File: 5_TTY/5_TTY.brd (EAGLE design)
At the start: 67.4 x 44.8 mm, 29 parts, among them Q2 BC857C, Q3 BC857C, Q4 BC857C, Q5 BC857C, Q6 BC857C, T4 BC847, X1 ALLSERIALSLAVE, X7 AKL18X-04W

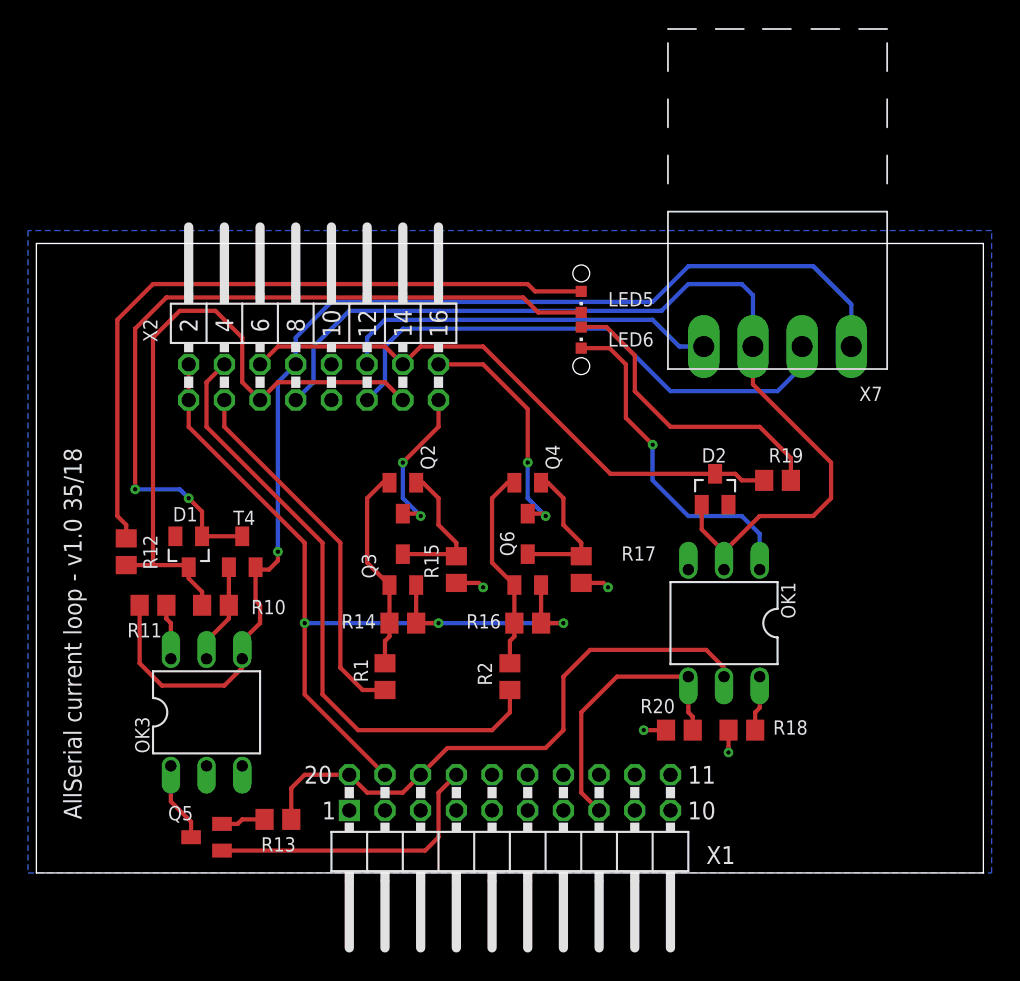
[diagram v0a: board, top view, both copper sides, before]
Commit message: final design & order
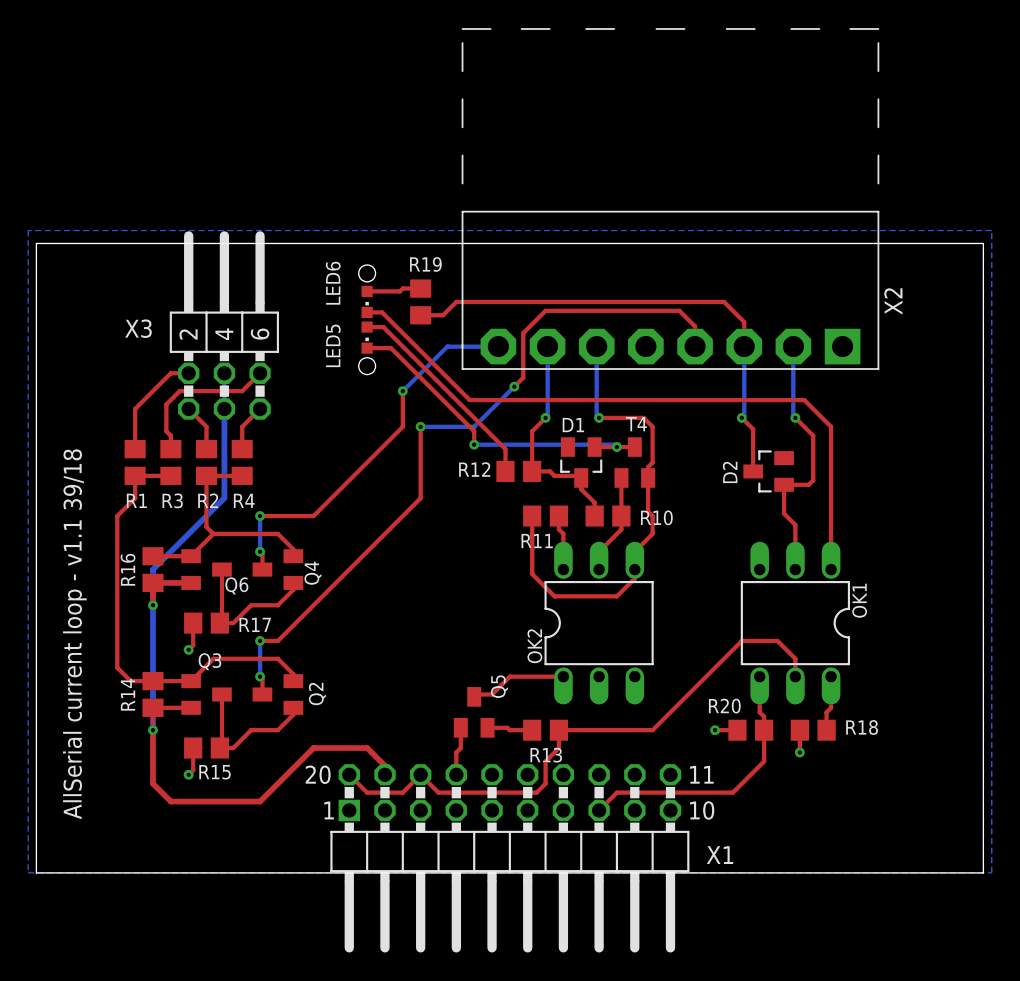
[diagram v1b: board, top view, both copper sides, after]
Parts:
- removed OK3: 4N25, optocoupler:DIL06
- removed X7: AKL18X-04W, con-riacon_akl:AKL182-04
- added OK2: 4N25, optocoupler:DIL06
- added R3, R4: 68R, resistor:R0805
- added X3: MA03-2W, con-lstb:MA03-2W
- R1, R2: value 33R -> 15R
- R14: value 33R -> 68R
- X2: value (none) -> AKL18X-08W; device con-lstb:MA08-2W -> con-riacon_akl:AKL182-08
- moved D1 28.7 mm to (39.4, 29.2)
- moved R10 28.7 mm to (41.3, 25.4)
- moved R11 28.7 mm to (36.8, 25.4)
- moved T4 28.7 mm to (43.2, 29.2)
- moved R12 28.5 mm to (34.9, 28.6), turned to 180 degrees
- moved R19 28.4 mm to (27.9, 40.6), turned to 90 degrees
- moved R16 26.9 mm to (8.89, 21.6), turned to 90 degrees
- moved R17 26.9 mm to (12.7, 17.8), turned to 0 degrees
- moved R2 26.4 mm to (12.7, 29.2), turned to 270 degrees
- moved X2 25.5 mm to (45.7, 37.5), turned to 180 degrees
- moved R1 23.4 mm to (7.62, 29.2), turned to 270 degrees
- moved Q6 22.9 mm to (12.7, 21.6), turned to 270 degrees
- moved R15 21.8 mm to (12.7, 8.89), turned to 0 degrees
- moved Q5 21.0 mm to (31.8, 11.4), turned to 0 degrees
- moved R13 20.1 mm to (36.8, 10.2)
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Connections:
- removed net CS1: R1.1, X2.3
- removed net CS2: R2.1, X2.4
- removed net N$44: X2.11, X7.P$2
- removed net N$65: X2.12, X7.P$4
- removed net RXN: D2.1, OK1.2, X2.7, X7.P$3
- removed net RXP: D2.3, R19.1, X2.14, X2.6
- removed net TXN: OK3.4, R11.2, T4.2, X2.8, X7.P$1
- new net N$2: R1.1, X3.2
- new net N$3: R2.1, X3.1
- new net N$4: OK2.4, R11.2, T4.2, X2.P$6
- new net N$5: R3.1, X3.6
- new net N$6: R4.1, X3.5
- new net N$7: D2.3, R19.1, X2.P$3
- new net N$8: D2.1, OK1.2, X2.P$2
- net +12V: now also X3.3, X3.4; no longer X2.1, X2.2
- net CC1: now also X2.P$4; no longer X2.15
- net CC2: now also X2.P$8; no longer X2.16
- net GND: now also OK2.2, X2.P$1, X2.P$5; no longer OK3.2, X2.10, X2.9
- net N$49: now also R4.2
- net N$54: now also OK2.6; no longer OK3.6
- net N$55: now also OK2.5; no longer OK3.5
- net N$59: now also R3.2
- net N$60: now also OK2.1; no longer OK3.1
- net TXP: now also X2.P$7; no longer X2.13, X2.5
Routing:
- net TXN: track 84.5 -> 0.00 mm, vias 1 -> 0
- net RXN: track 69.0 -> 0.00 mm
- net CS2: track 43.9 -> 0.00 mm
- net RXP: track 41.4 -> 0.00 mm
- net CC1: track 11.2 -> 51.3 mm, vias 2 -> 4
- net N$44: track 38.5 -> 0.00 mm
- net N$58: track 50.1 -> 15.0 mm
- net N$7: track 0.00 -> 35.0 mm, vias 0 -> 1
- net N$4: track 0.00 -> 33.7 mm, vias 0 -> 1
- net TXP: track 47.9 -> 16.1 mm, vias 0 -> 1
- net N$56: track 54.6 -> 24.1 mm
- net N$65: track 27.2 -> 0.00 mm
- net CS1: track 26.3 -> 0.00 mm
- net N$63: track 24.4 -> 46.6 mm, vias 1 -> 0
- net N$8: track 0.00 -> 18.7 mm, vias 0 -> 1
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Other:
- board text added: "AllSerial current loop - v1.1 39/18"
- board text removed: "AllSerial current loop - v1.0 35/18"
